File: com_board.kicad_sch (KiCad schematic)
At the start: 32 parts, among them IC1 nRF52820-QDAA-R, J1 USB_C_Receptacle_USB2.0_16P, J2 Conn_ST_STDC14, J3 U.FL-R-SMT_01_, U2 USBLC6-2SC6, Y1 32.768kHz Cl=9pF, Y2 32MHz Cl=8pF

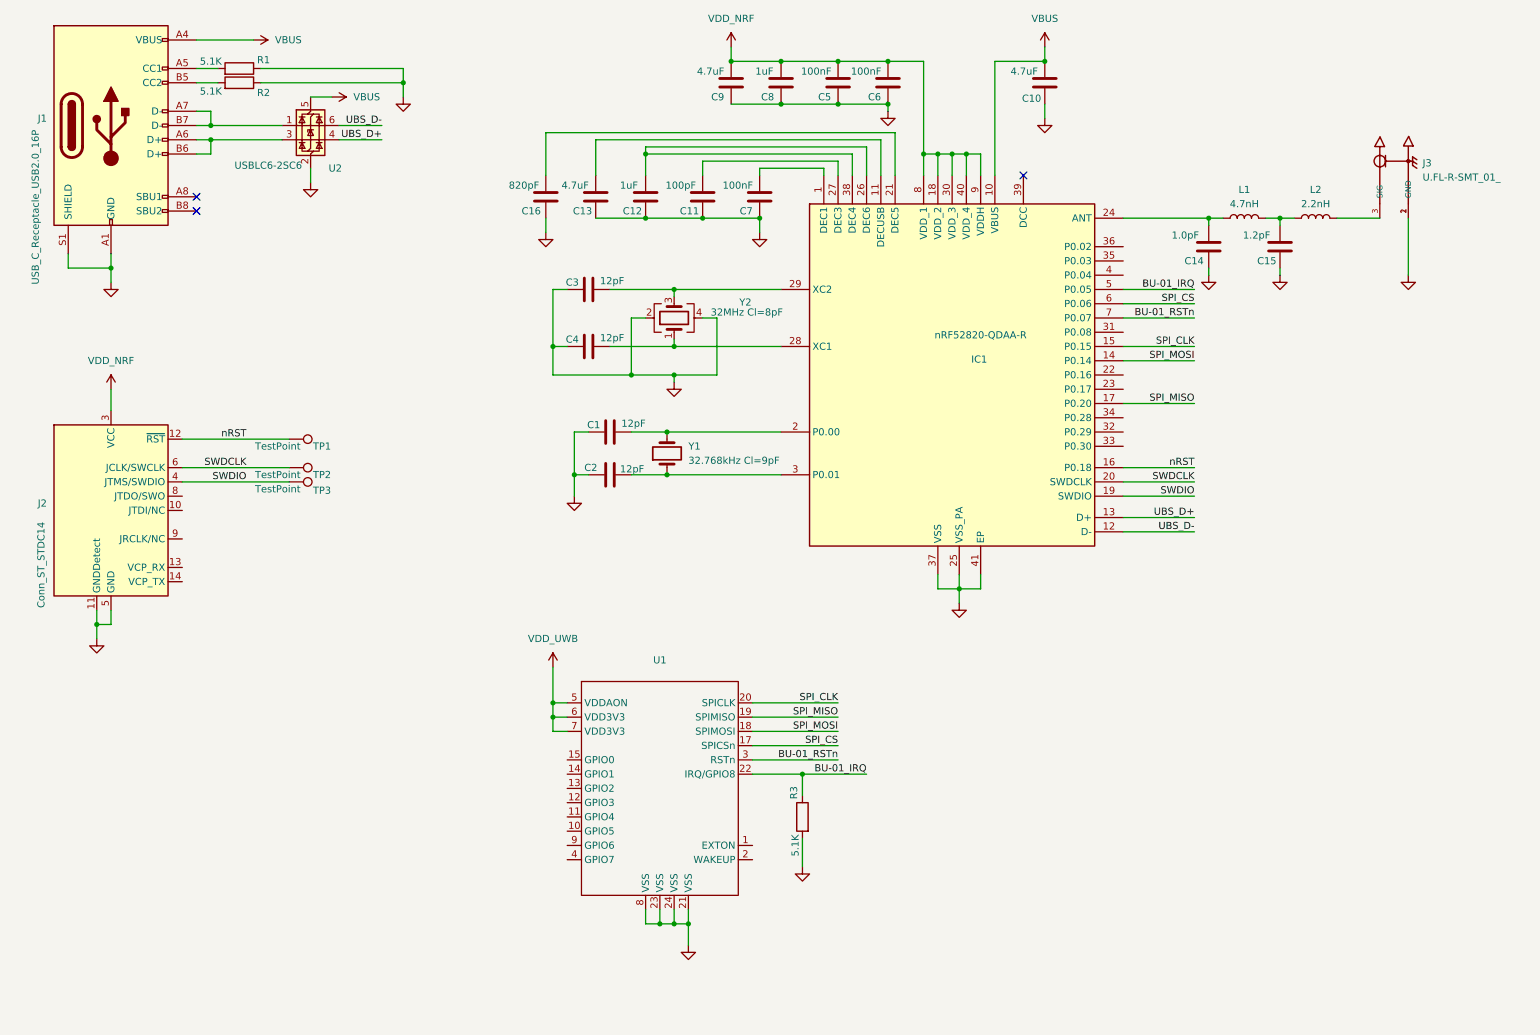
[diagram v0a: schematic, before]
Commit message: Finished schematic
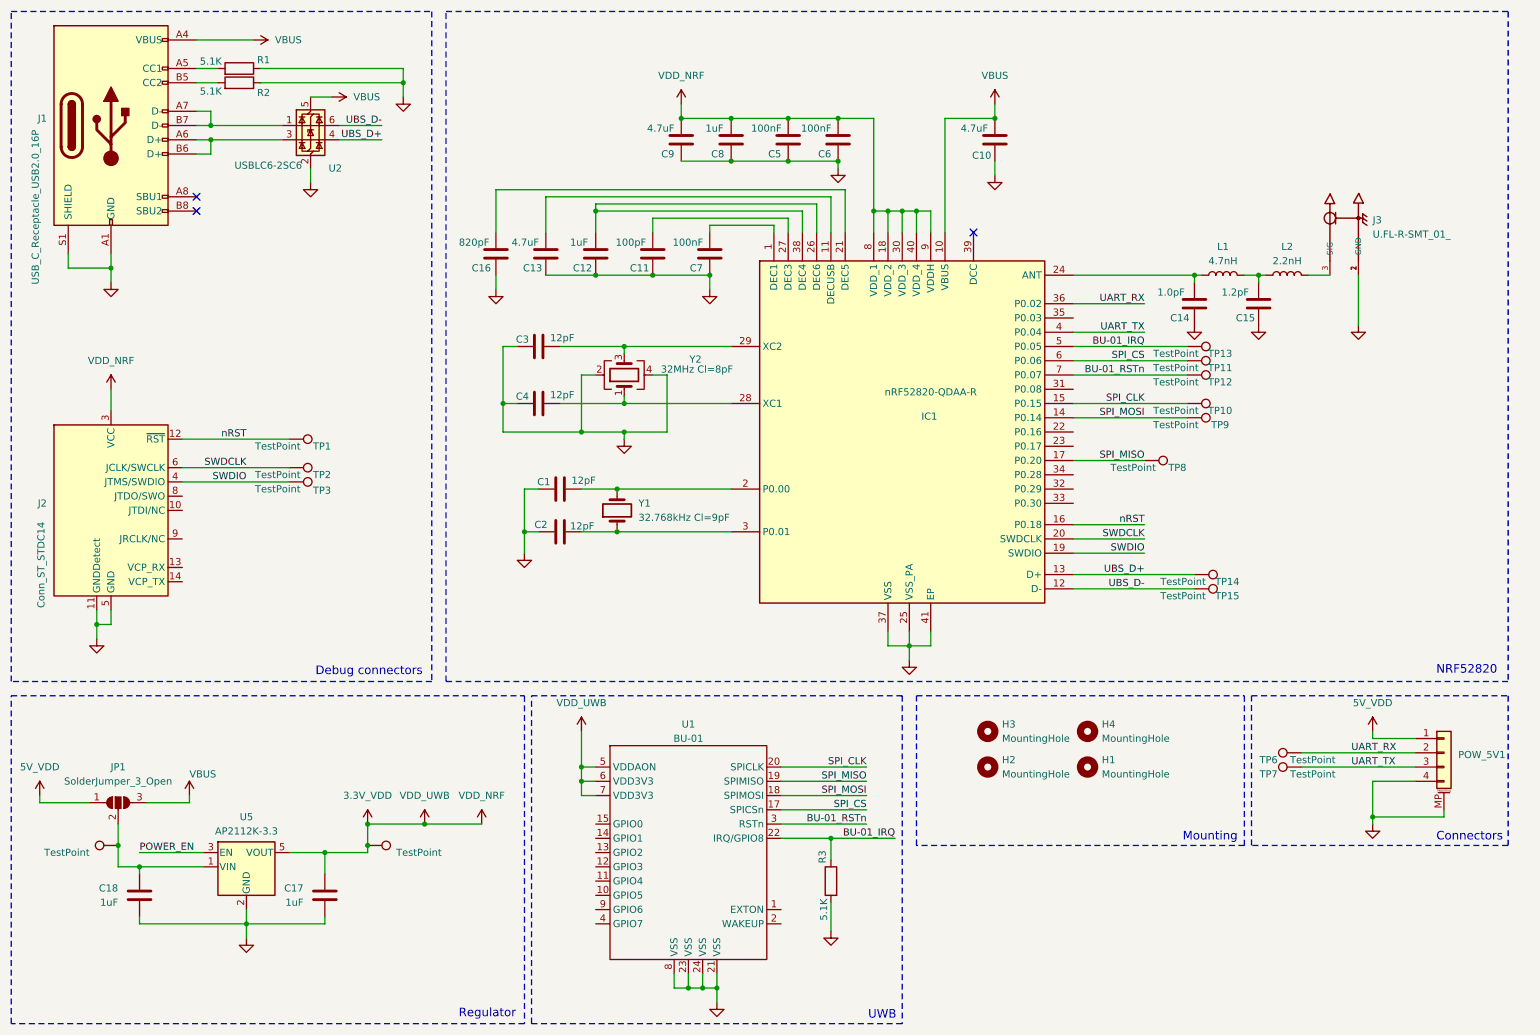
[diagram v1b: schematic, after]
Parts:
- added C17, C18: 1uF, Capacitor_SMD:C_0402_1005Metric_Pad0.74x0.62mm_HandSolder, symbol Device:C
- added H1, H2, H3, H4: MountingHole, MountingHole:MountingHole_2.2mm_M2, symbol Mechanical:MountingHole
- added JP1: SolderJumper_3_Open, Jumper:SolderJumper-3_P1.3mm_Open_Pad1.0x1.5mm_NumberLabels, symbol Jumper:SolderJumper_3_Open
- added POW_5V1: FFC-FPC:TE_84952_4, Connector_FFC-FPC:TE_84952-4_1x04-1MP_P1.0mm_Horizontal, symbol Connector_Generic_MountingPin:Conn_01x04_MountingPin
- added TP10, TP11, TP12, TP13, TP14, TP15, TP4, TP5, TP6, TP7, TP8, TP9: TestPoint, TestPoint:TestPoint_Pad_D1.0mm, symbol Connector:TestPoint
- added U5: AP2112K-3.3, Package_TO_SOT_SMD:SOT-23-5, symbol Regulator_Linear:AP2112K-3.3
- IC1: footprint QFN40P500X500X90-41N-D -> NRF52qdaa:QFN40P500X500X90-41N-D
- U1: value ~ -> BU-01; footprint (none) -> bu-01:BU-01
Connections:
- net VDD_UWB is gone; now on net 3.3V_VDD: U1.5 (VDDAON), U1.6 (VDD3V3), U1.7 (VDD3V3)
- net BU-01_IRQ: now also TP13.1
- net BU-01_RSTn: now also TP12.1
- net GND: now also C17.2, C18.2, POW_5V1.4 (Pin_4), POW_5V1.MP (MountPin), U5.2 (GND)
- net SPI_CLK: now also TP10.1
- net SPI_CS: now also TP11.1
- net SPI_MISO: now also TP8.1
- net SPI_MOSI: now also TP9.1
- net UBS_D+: now also TP14.1
- net UBS_D-: now also TP15.1
- net VBUS: now also JP1.3 (B)
- net UART_RX: now reaches IC1.36 (P0.02)
- net UART_RX: now also POW_5V1.2 (Pin_2), TP6.1
- net UART_TX: now reaches IC1.4 (P0.04)
- net UART_TX: now also POW_5V1.3 (Pin_3), TP7.1
- net VDD_NRF renamed 3.3V_VDD
- net 3.3V_VDD: now also C17.1, TP4.1, U5.5 (VOUT)
- new net: C18.1, JP1.2 (C), TP5.1, U5.1 (VIN)
- new net 5V_VDD: JP1.1 (A), POW_5V1.1 (Pin_1)
- new net POWER_EN: U5.3 (EN)
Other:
- note added: "Connectors"
- note added: "Debug connectors"
- note added: "Mounting"
- note added: "NRF52820"
- note added: "Regulator"
- note added: "UWB"
- moved on the sheet: C1, C10, C11, C12, C13, C14, C15, C16, C2, C3, C4, C5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
